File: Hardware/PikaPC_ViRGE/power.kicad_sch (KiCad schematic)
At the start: 27 parts, among them U1 86C325, U2 ATF1504AS

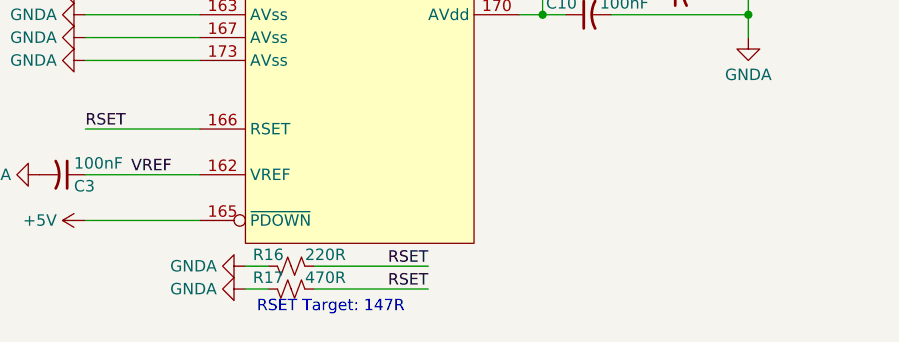
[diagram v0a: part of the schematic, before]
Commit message: Prep for output
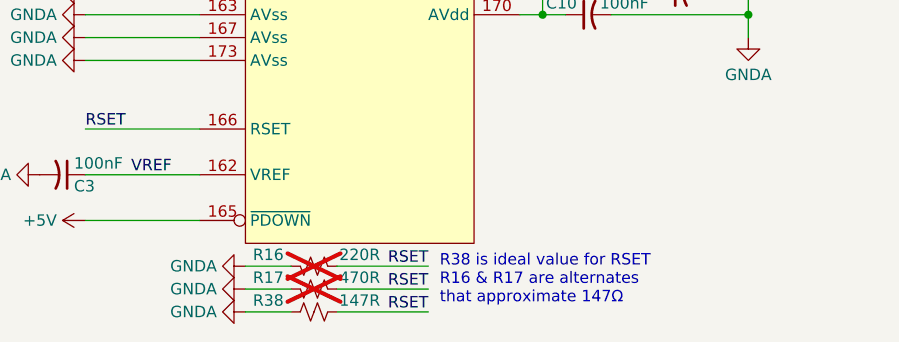
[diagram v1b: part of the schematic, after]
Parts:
- added R38: 147R, Resistor_SMD:R_0805_2012Metric, symbol Device:R_Small_US
- C10, C11, C12, C13, C14, C15, C19, C20, C21, C3, C4, C48, C5, C6, C7, C8, C9: Mouser (none) -> 187-CL21B104KACNNNC
- C16, C17, C22: Mouser (none) -> 187-CL21B105KOFNNNG
- L1, L2: Mouser (none) -> 708-RMCF1210ZT0R00
- R16, R17: now not fitted
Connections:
- net GNDA: now also R38.1
- net RSET: now also R38.2
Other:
- note added: "R38 is ideal value for RSET R16 & R17 are alternates that approximate 147Ω"
- note removed: "RSET Target: 147R"
